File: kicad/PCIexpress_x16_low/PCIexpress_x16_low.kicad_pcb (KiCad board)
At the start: 4 copper layers, 167.7 x 68.9 mm, 66 parts, among them J1 PCIexpress_bracket, J2 PCIexpress_x16

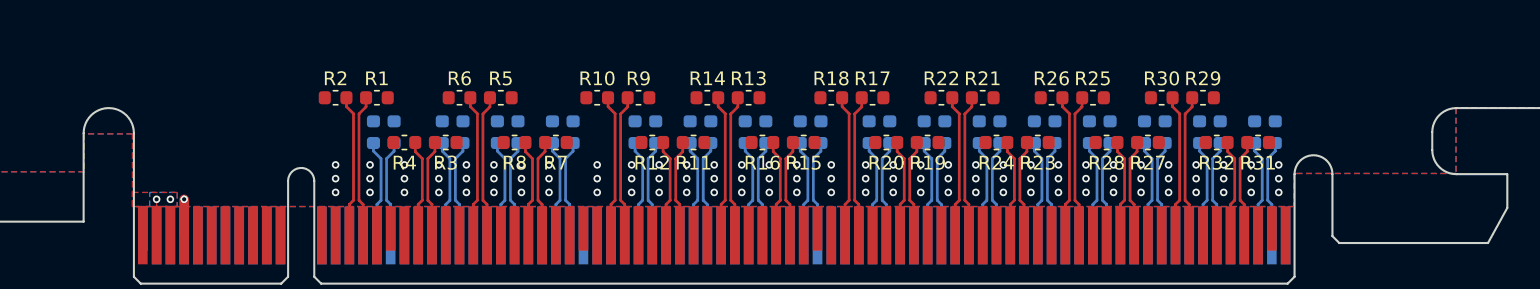
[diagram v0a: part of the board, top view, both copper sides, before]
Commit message: test
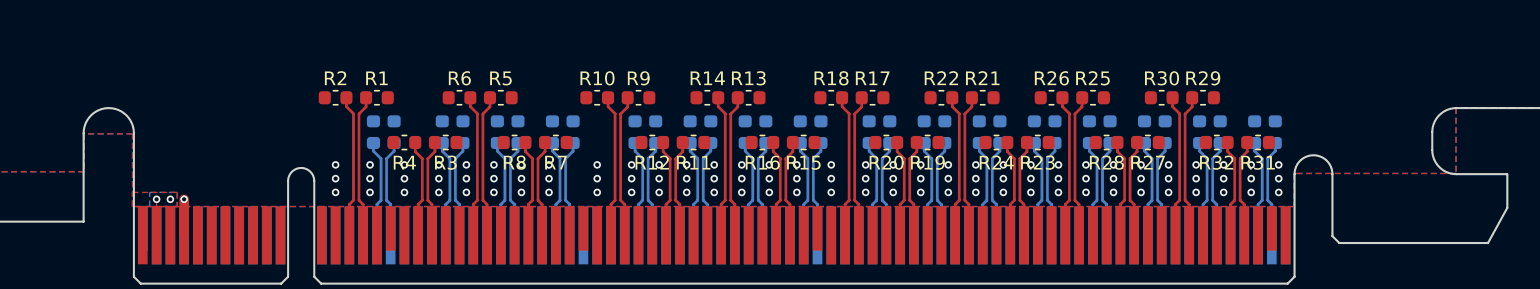
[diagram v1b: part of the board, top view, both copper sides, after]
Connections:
- net /~PERST renamed /~{PERST}
- net /~PRSNT1 renamed /~{PRSNT1}
- net /~PRSNT2x1 renamed /~{PRSNT2x1}
- net /~PRSNT2x16 renamed /~{PRSNT2x16}
- net /~PRSNT2x4 renamed /~{PRSNT2x4}
- net /~PRSNT2x8 renamed /~{PRSNT2x8}
- net /~TRST renamed /~{TRST}
- net /~WAKE renamed /~{WAKE}
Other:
- net class Default removed
- net class Diff-100-PCIe removed
- net class JLC2313-100d-3.5 removed
- net class JLC2313-100d-4 removed
- net class JLC7628-100d-8 removed
